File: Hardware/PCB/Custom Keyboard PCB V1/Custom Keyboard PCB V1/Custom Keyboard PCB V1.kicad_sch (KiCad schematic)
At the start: 5 parts, among them SW1 RotaryEncoder_Switch_MP, U1 WeMos_S3_mini

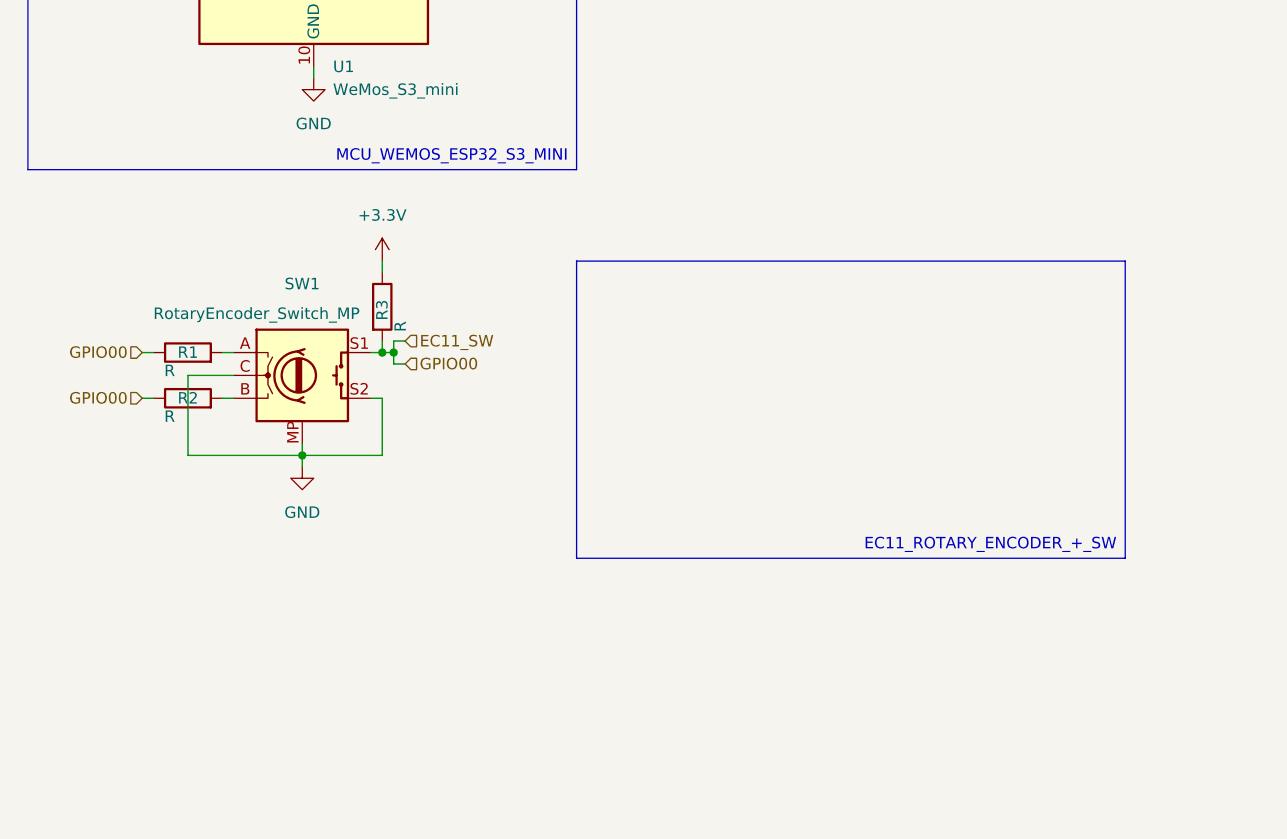
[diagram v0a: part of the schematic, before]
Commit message: uhhhhhhhhhhhhhhh
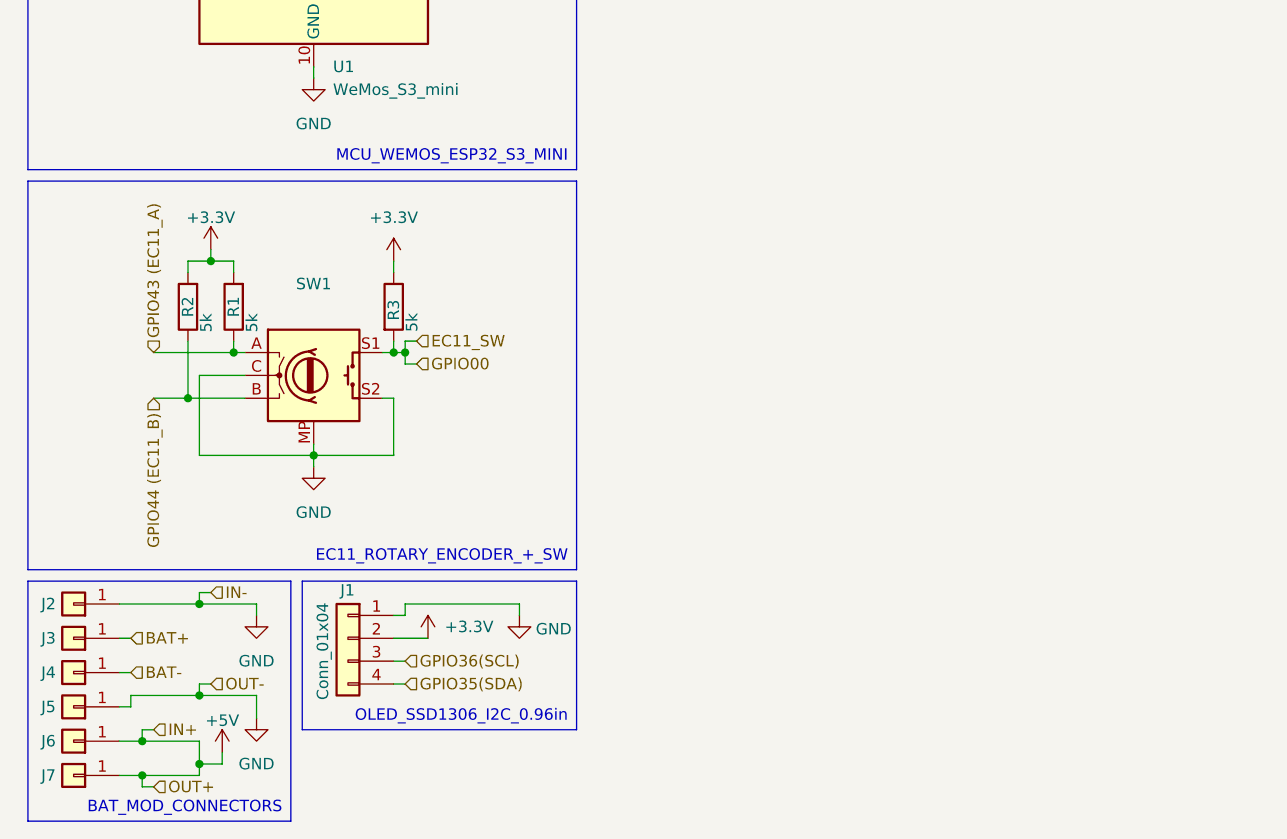
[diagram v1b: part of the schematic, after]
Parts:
- added J1: Conn_01x04, Wireless Keyboard:OLED_SSD1306_I2C_0.96, symbol Connector_Generic:Conn_01x04
- added J2, J5, J6, J7: Conn_01x01, Connector_PinHeader_2.54mm:PinHeader_1x01_P2.54mm_Vertical, symbol Connector_Generic:Conn_01x01
- added J3, J4: Conn_01x01, symbol Connector_Generic:Conn_01x01
- R1, R2: value R -> 5k
- R3: value R -> 5k; footprint (none) -> Resistor_THT:R_Axial_DIN0204_L3.6mm_D1.6mm_P5.08mm_Horizontal
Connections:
- net +3.3V: now also R1.2, R2.2, J1.2 (Pin_2)
- net +5V: now also J6.1 (Pin_1), J7.1 (Pin_1)
- net EC11_SW: no longer R1.1, R2.1
- net GND: now also J1.1 (Pin_1), J2.1 (Pin_1), J5.1 (Pin_1)
- net GPIO35(SDA): now also J1.4 (Pin_4)
- net GPIO36(SCL): now also J1.3 (Pin_3)
- net GPIO43 (EC11_A): now reaches SW1.A
- net GPIO43 (EC11_A): now also R1.1; no longer R1.2
- net GPIO44 (EC11_B): now reaches SW1.B
- net GPIO44 (EC11_B): now also R2.1; no longer R2.2
- new net BAT+: J3.1 (Pin_1)
- new net BAT-: J4.1 (Pin_1)
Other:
- moved on the sheet: R3, SW1

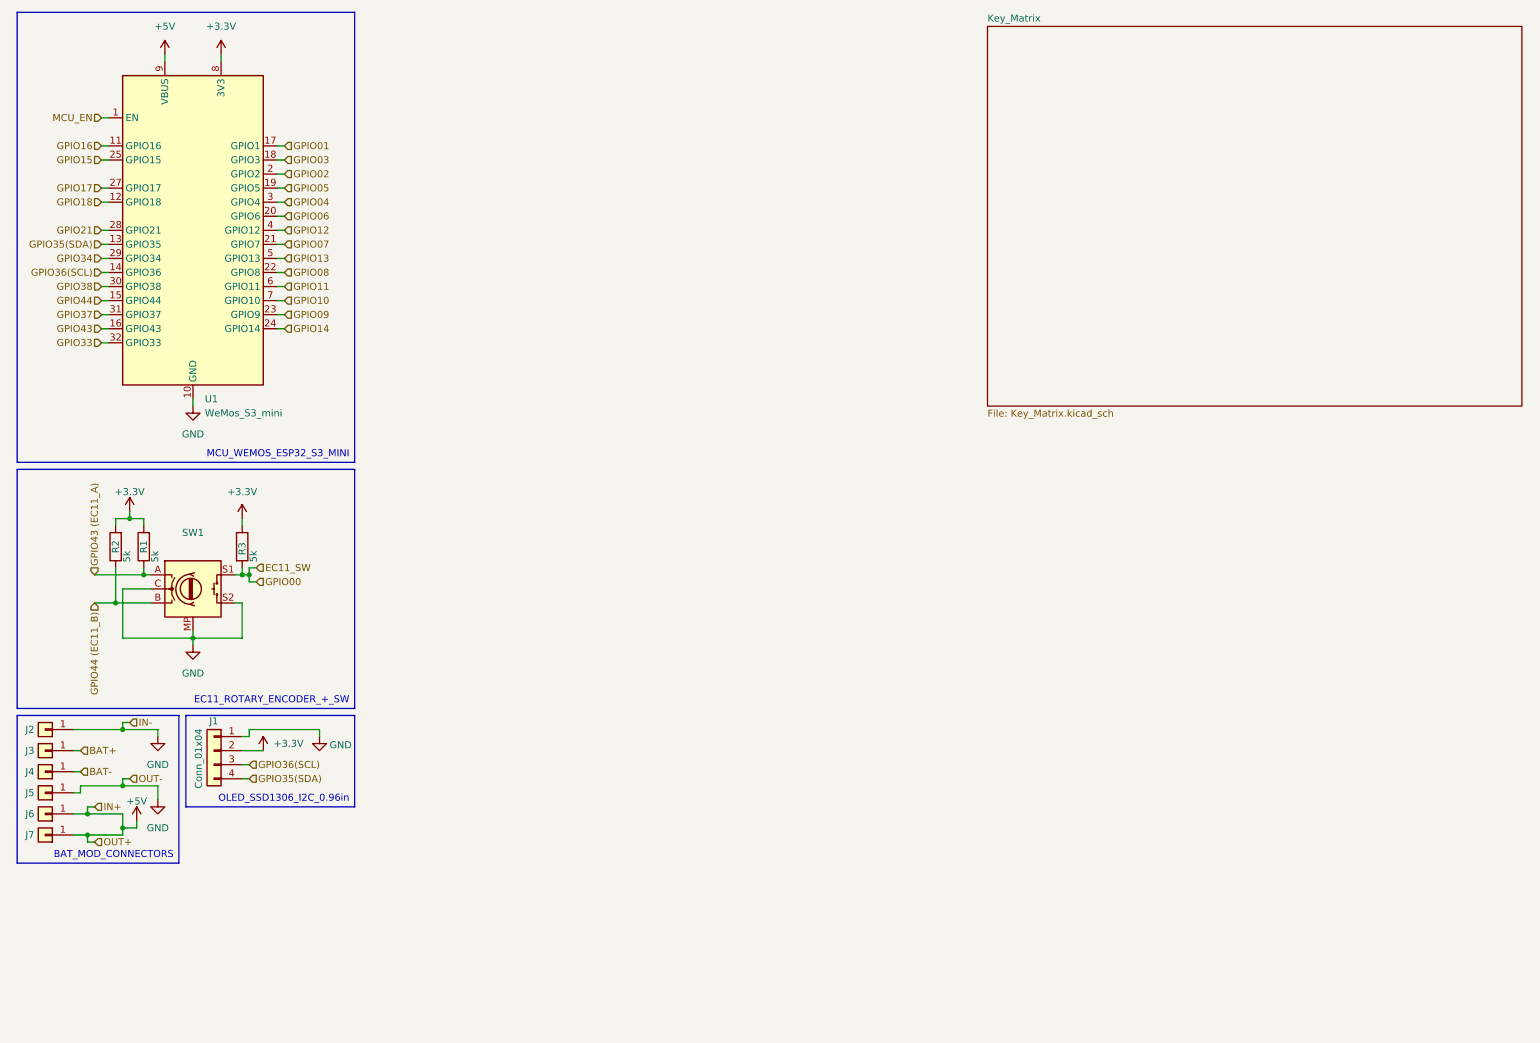
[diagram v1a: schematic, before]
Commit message: uhhhhhhhhhhhhhhhhhhhhhhhhhhhhhhhhhhhhh
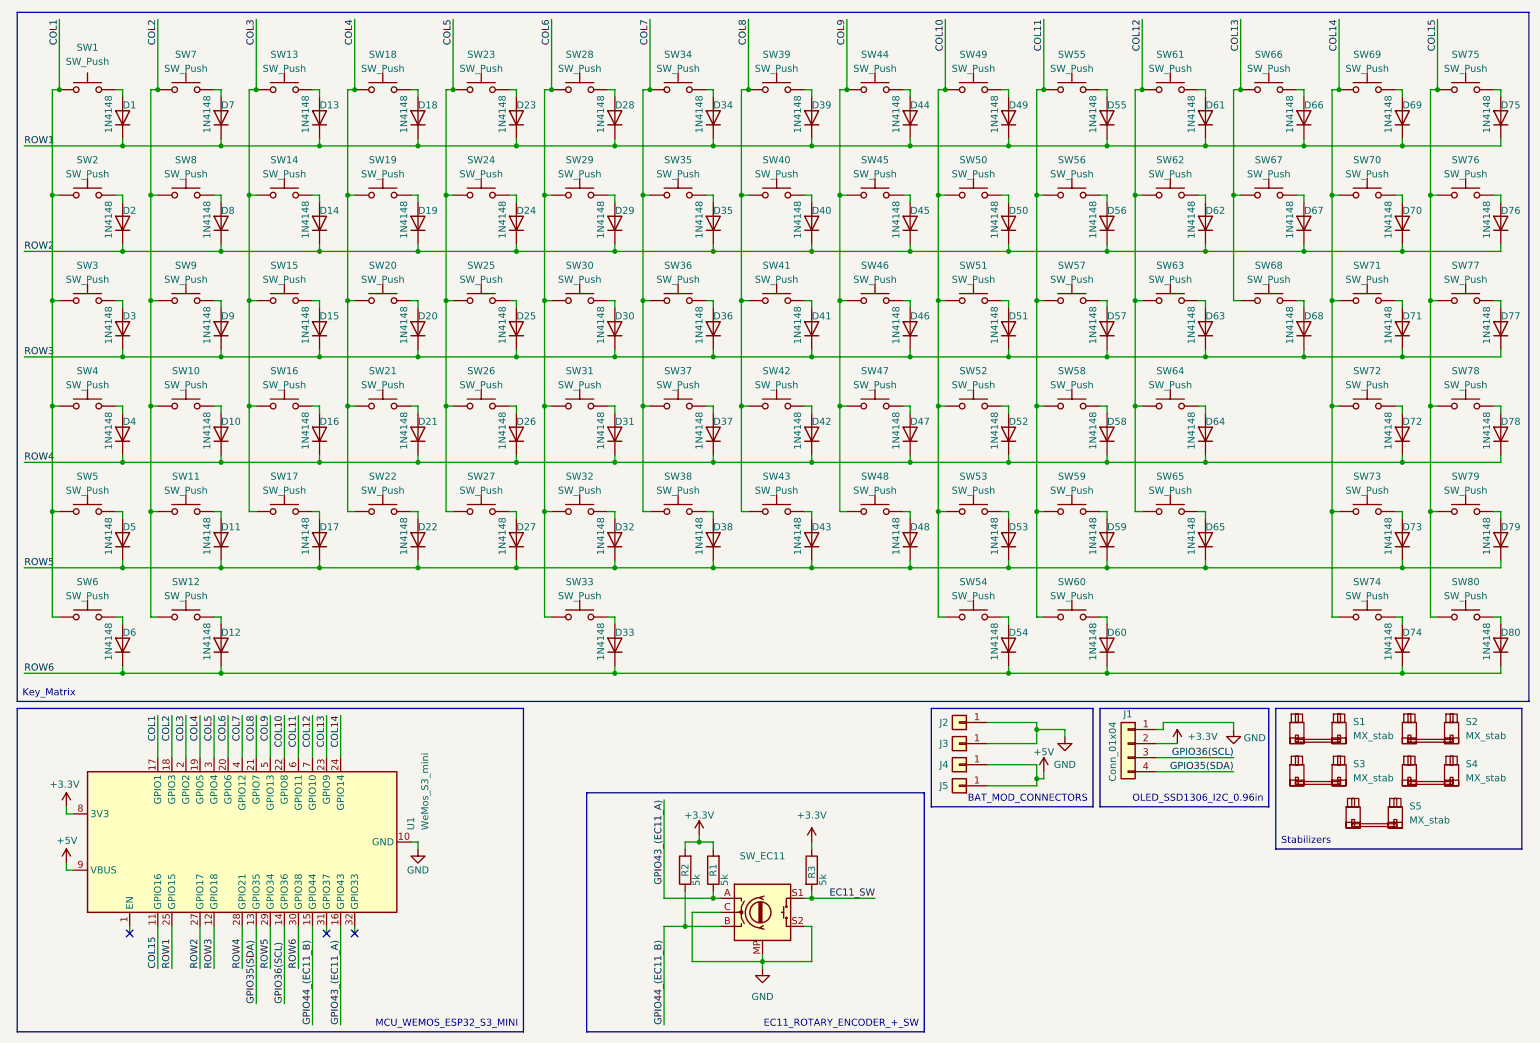
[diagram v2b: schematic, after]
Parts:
- removed J3, J4: Conn_01x01, symbol Connector_Generic:Conn_01x01
- added D1, D10, D11, D12, D13, D14, D15, D16, D17, D18, D19, D2, D20, D21, D22, D23, D24, D25, D26, D27, D28, D29, D3, D30, D31, D32, D33, D34, D35, D36, D37, D38, D39, D4, D40, D41, D42, D43, D44, D45, D46, D47, D48, D49, D5, D50, D51, D52, D53, D54, D55, D56, D57, D58, D59, D6, D60, D61, D62, D63, D64, D65, D66, D67, D68, D69, D7, D70, D71, D72, D73, D74, D75, D76, D77, D78, D79, D8, D80, D9: 1N4148, Diode_SMD:D_MiniMELF_Handsoldering, symbol Device:D
- added S1, S2, S3, S4: MX_stab, PCM_marbastlib-mx:STAB_MX_P_2u, symbol marbastlib-mx:MX_stab
- added S5: MX_stab, PCM_marbastlib-mx:STAB_MX_P_6.25u, symbol marbastlib-mx:MX_stab
- added SW1, SW10, SW11, SW12, SW13, SW14, SW15, SW16, SW17, SW18, SW19, SW2, SW20, SW21, SW22, SW23, SW24, SW25, SW26, SW27, SW28, SW29, SW3, SW30, SW31, SW32, SW33, SW34, SW35, SW36, SW37, SW38, SW39, SW4, SW40, SW41, SW42, SW43, SW44, SW45, SW46, SW47, SW48, SW49, SW5, SW50, SW51, SW52, SW53, SW54, SW55, SW56, SW57, SW58, SW59, SW6, SW60, SW61, SW62, SW63, SW64, SW65, SW66, SW67, SW68, SW69, SW7, SW70, SW71, SW72, SW73, SW74, SW75, SW76, SW77, SW78, SW79, SW8, SW80, SW9: SW_Push, PCM_marbastlib-mx:SW_MX_1u, symbol Switch:SW_Push
- renumbered J5 to J3, J6 to J4, J7 to J5, SW1 to SW_EC11
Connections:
- net GPIO43 (EC11_A) is gone; now on net GPIO43_(EC11_A): R1.1, SW_EC11.A
- net GPIO44 (EC11_B) is gone; now on net GPIO44_(EC11_B): R2.1, SW_EC11.B
- net GPIO01 renamed COL1
- net COL1: now also SW1.1, SW2.1, SW3.1, SW4.1, SW5.1, SW6.1
- net GPIO02 renamed COL3
- net COL3: now also SW13.1, SW14.1, SW15.1, SW16.1, SW17.1
- net GPIO03 renamed COL2
- net COL2: now also SW10.1, SW11.1, SW12.1, SW7.1, SW8.1, SW9.1
- net GPIO04 renamed COL5
- net COL5: now also SW23.1, SW24.1, SW25.1, SW26.1, SW27.1
- net GPIO05 renamed COL4
- net COL4: now also SW18.1, SW19.1, SW20.1, SW21.1, SW22.1
- net GPIO06 renamed COL6
- net COL6: now also SW28.1, SW29.1, SW30.1, SW31.1, SW32.1, SW33.1
- net GPIO07 renamed COL8
- net COL8: now also SW39.1, SW40.1, SW41.1, SW42.1, SW43.1
- net GPIO08 renamed COL10
- net COL10: now also SW49.1, SW50.1, SW51.1, SW52.1, SW53.1, SW54.1
- net GPIO09 renamed COL13
- net COL13: now also SW66.1, SW67.1, SW68.1
- net GPIO10 renamed COL12
- net COL12: now also SW61.1, SW62.1, SW63.1, SW64.1, SW65.1
- net GPIO11 renamed COL11
- net COL11: now also SW55.1, SW56.1, SW57.1, SW58.1, SW59.1, SW60.1
- net GPIO12 renamed COL7
- net COL7: now also SW34.1, SW35.1, SW36.1, SW37.1, SW38.1
- net GPIO13 renamed COL9
- net COL9: now also SW44.1, SW45.1, SW46.1, SW47.1, SW48.1
- net GPIO14 renamed COL14
- net COL14: now also SW69.1, SW70.1, SW71.1, SW72.1, SW73.1, SW74.1
- net GPIO15 renamed ROW1
- net ROW1: now also D1.1 (K), D13.1 (K), D18.1 (K), D23.1 (K), D28.1 (K), D34.1 (K), D39.1 (K), D44.1 (K), D49.1 (K), D55.1 (K), D61.1 (K), D66.1 (K), D69.1 (K), D7.1 (K), D75.1 (K)
- net GPIO16 renamed COL15
- net COL15: now also SW75.1, SW76.1, SW77.1, SW78.1, SW79.1, SW80.1
- net GPIO17 renamed ROW2
- net ROW2: now also D14.1 (K), D19.1 (K), D2.1 (K), D24.1 (K), D29.1 (K), D35.1 (K), D40.1 (K), D45.1 (K), D50.1 (K), D56.1 (K), D62.1 (K), D67.1 (K), D70.1 (K), D76.1 (K), D8.1 (K)
- net GPIO18 renamed ROW3
- net ROW3: now also D15.1 (K), D20.1 (K), D25.1 (K), D3.1 (K), D30.1 (K), D36.1 (K), D41.1 (K), D46.1 (K), D51.1 (K), D57.1 (K), D63.1 (K), D68.1 (K), D71.1 (K), D77.1 (K), D9.1 (K)
- net GPIO21 renamed ROW4
- net ROW4: now also D10.1 (K), D16.1 (K), D21.1 (K), D26.1 (K), D31.1 (K), D37.1 (K), D4.1 (K), D42.1 (K), D47.1 (K), D52.1 (K), D58.1 (K), D64.1 (K), D72.1 (K), D78.1 (K)
- net GPIO33: no longer names the net of U1.32 (GPIO33)
- net GPIO34 renamed ROW5
- net ROW5: now also D11.1 (K), D17.1 (K), D22.1 (K), D27.1 (K), D32.1 (K), D38.1 (K), D43.1 (K), D48.1 (K), D5.1 (K), D53.1 (K), D59.1 (K), D65.1 (K), D73.1 (K), D79.1 (K)
- net GPIO37: no longer names the net of U1.31 (GPIO37)
- net GPIO38 renamed ROW6
- net ROW6: now also D12.1 (K), D33.1 (K), D54.1 (K), D6.1 (K), D60.1 (K), D74.1 (K), D80.1 (K)
- net GPIO43 renamed GPIO43_(EC11_A)
- net GPIO44 renamed GPIO44_(EC11_B)
- net MCU_EN: no longer names the net of U1.1 (EN)
- new net: D66.2 (A), SW66.2
- new net: D37.2 (A), SW37.2
- new net: D47.2 (A), SW47.2
- new net: D78.2 (A), SW78.2
- new net: D1.2 (A), SW1.2
- new net: D7.2 (A), SW7.2
- new net: D36.2 (A), SW36.2
- new net: D35.2 (A), SW35.2
- new net: D72.2 (A), SW72.2
- new net: D50.2 (A), SW50.2
- new net: D45.2 (A), SW45.2
- new net: D14.2 (A), SW14.2
- new net: D11.2 (A), SW11.2
- new net: D43.2 (A), SW43.2
- new net: D29.2 (A), SW29.2
- new net: D21.2 (A), SW21.2
- new net: D69.2 (A), SW69.2
- new net: D24.2 (A), SW24.2
- new net: D28.2 (A), SW28.2
- new net: D74.2 (A), SW74.2
- new net: D59.2 (A), SW59.2
- new net: D9.2 (A), SW9.2
- new net: D40.2 (A), SW40.2
- new net: D80.2 (A), SW80.2
- new net: D58.2 (A), SW58.2
- new net: D62.2 (A), SW62.2
- new net: D31.2 (A), SW31.2
- new net: D3.2 (A), SW3.2
- new net: D79.2 (A), SW79.2
- new net: D16.2 (A), SW16.2
- new net: D10.2 (A), SW10.2
- new net: D23.2 (A), SW23.2
- new net: D46.2 (A), SW46.2
- new net: D12.2 (A), SW12.2
- new net: D60.2 (A), SW60.2
- new net: D34.2 (A), SW34.2
- new net: D33.2 (A), SW33.2
- new net: D26.2 (A), SW26.2
- new net: D70.2 (A), SW70.2
- new net: D48.2 (A), SW48.2
- new net: D51.2 (A), SW51.2
- new net: D25.2 (A), SW25.2
- new net: D54.2 (A), SW54.2
- new net: D53.2 (A), SW53.2
- new net: D77.2 (A), SW77.2
- new net: D63.2 (A), SW63.2
- new net: D75.2 (A), SW75.2
- new net: D17.2 (A), SW17.2
- new net: D71.2 (A), SW71.2
- new net: D44.2 (A), SW44.2
- new net: D6.2 (A), SW6.2
- new net: D20.2 (A), SW20.2
- new net: D67.2 (A), SW67.2
- new net: D52.2 (A), SW52.2
- new net: D19.2 (A), SW19.2
- new net: D56.2 (A), SW56.2
- new net: D65.2 (A), SW65.2
- new net: D32.2 (A), SW32.2
- new net: D30.2 (A), SW30.2
- new net: D27.2 (A), SW27.2
- new net: D68.2 (A), SW68.2
- new net: D15.2 (A), SW15.2
- new net: D2.2 (A), SW2.2
- new net: D49.2 (A), SW49.2
- new net: D64.2 (A), SW64.2
- new net: D61.2 (A), SW61.2
- new net: D42.2 (A), SW42.2
- new net: D18.2 (A), SW18.2
- new net: D55.2 (A), SW55.2
- new net: D41.2 (A), SW41.2
- new net: D4.2 (A), SW4.2
- new net: D8.2 (A), SW8.2
- new net: D38.2 (A), SW38.2
- new net: D13.2 (A), SW13.2
- new net: D76.2 (A), SW76.2
- new net: D5.2 (A), SW5.2
- new net: D22.2 (A), SW22.2
- new net: D57.2 (A), SW57.2
- new net: D39.2 (A), SW39.2
- new net: D73.2 (A), SW73.2
- no-connect marks 0 -> 3
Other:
- removed sheet Key_Matrix
- moved on the sheet: J1, J2, J3, J4, J5, R1, R2, R3, SW_EC11, U1

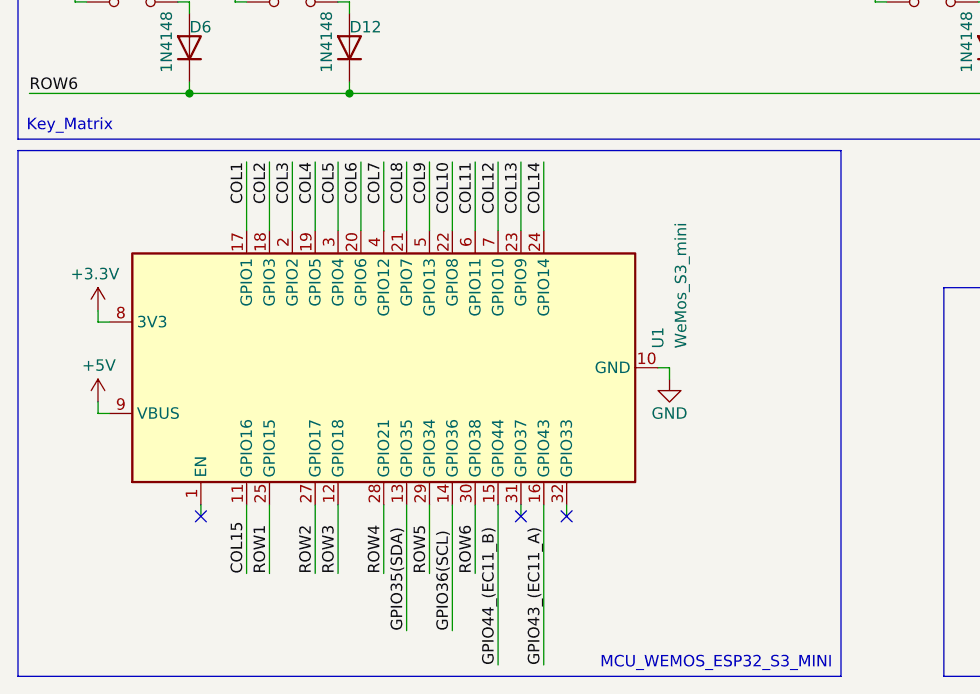
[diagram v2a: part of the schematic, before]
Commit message: might be broken
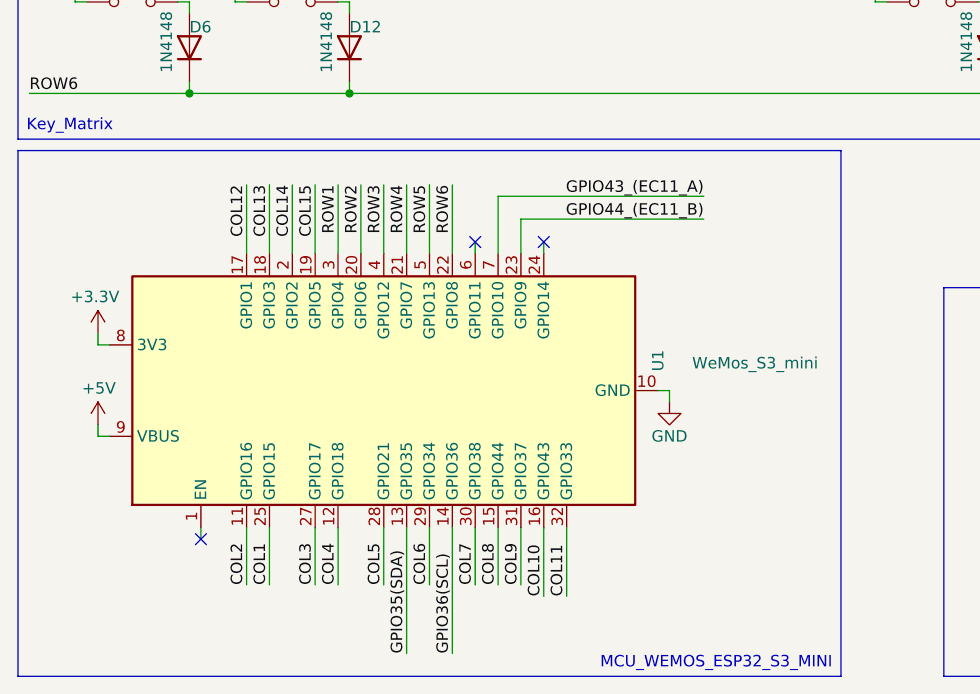
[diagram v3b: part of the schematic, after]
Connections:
- net COL1: now also U1.25 (GPIO15); no longer U1.17 (GPIO1)
- net COL10: now also U1.16 (GPIO43); no longer U1.22 (GPIO8)
- net COL11: now also U1.32 (GPIO33); no longer U1.6 (GPIO11)
- net COL12: now also U1.17 (GPIO1); no longer U1.7 (GPIO10)
- net COL13: now also U1.18 (GPIO3); no longer U1.23 (GPIO9)
- net COL14: now also U1.2 (GPIO2); no longer U1.24 (GPIO14)
- net COL15: now also U1.19 (GPIO5); no longer U1.11 (GPIO16)
- net COL2: now also U1.11 (GPIO16); no longer U1.18 (GPIO3)
- net COL3: now also U1.27 (GPIO17); no longer U1.2 (GPIO2)
- net COL4: now also U1.12 (GPIO18); no longer U1.19 (GPIO5)
- net COL5: now also U1.28 (GPIO21); no longer U1.3 (GPIO4)
- net COL6: now also U1.29 (GPIO34); no longer U1.20 (GPIO6)
- net COL7: now also U1.30 (GPIO38); no longer U1.4 (GPIO12)
- net COL8: now also U1.15 (GPIO44); no longer U1.21 (GPIO7)
- net COL9: now also U1.31 (GPIO37); no longer U1.5 (GPIO13)
- net GPIO43_(EC11_A): now also U1.7 (GPIO10); no longer U1.16 (GPIO43)
- net GPIO44_(EC11_B): now also U1.23 (GPIO9); no longer U1.15 (GPIO44)
- net ROW1: now also U1.3 (GPIO4); no longer U1.25 (GPIO15)
- net ROW2: now also U1.20 (GPIO6); no longer U1.27 (GPIO17)
- net ROW3: now also U1.4 (GPIO12); no longer U1.12 (GPIO18)
- net ROW4: now also U1.21 (GPIO7); no longer U1.28 (GPIO21)
- net ROW5: now also U1.5 (GPIO13); no longer U1.29 (GPIO34)
- net ROW6: now also U1.22 (GPIO8); no longer U1.30 (GPIO38)
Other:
- moved on the sheet: U1
